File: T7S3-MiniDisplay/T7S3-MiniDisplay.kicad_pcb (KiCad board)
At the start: 2 copper layers, 67.3 x 63.5 mm, 37 parts, among them J101 Qwicc, J102 Micro_SD_Card_Det, J801 RJ45, J802 RJ45, T801 + 15 in -, T802 + 15 out -, U101 TTGO-T7_S3-V1.1, U301 AP63205, U801 TCAN332DR

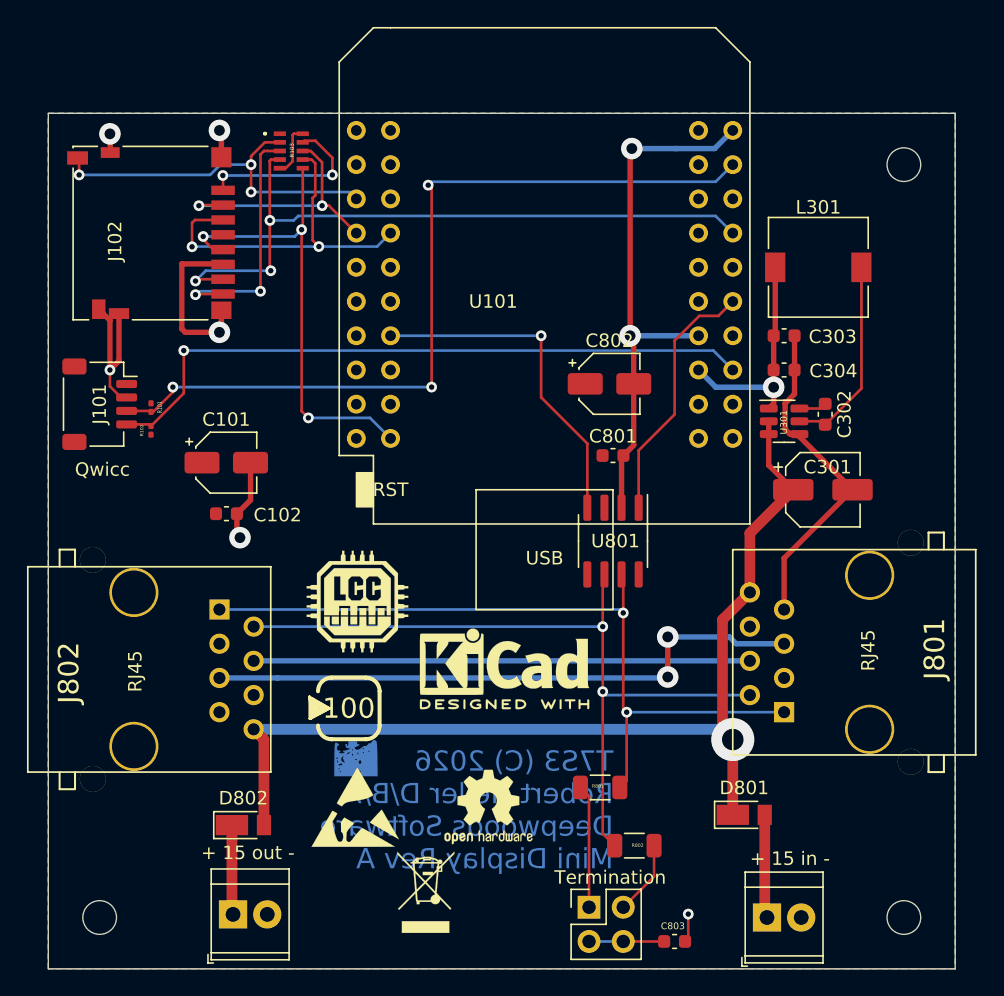
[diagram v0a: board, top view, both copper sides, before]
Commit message: Finalize part numbers.
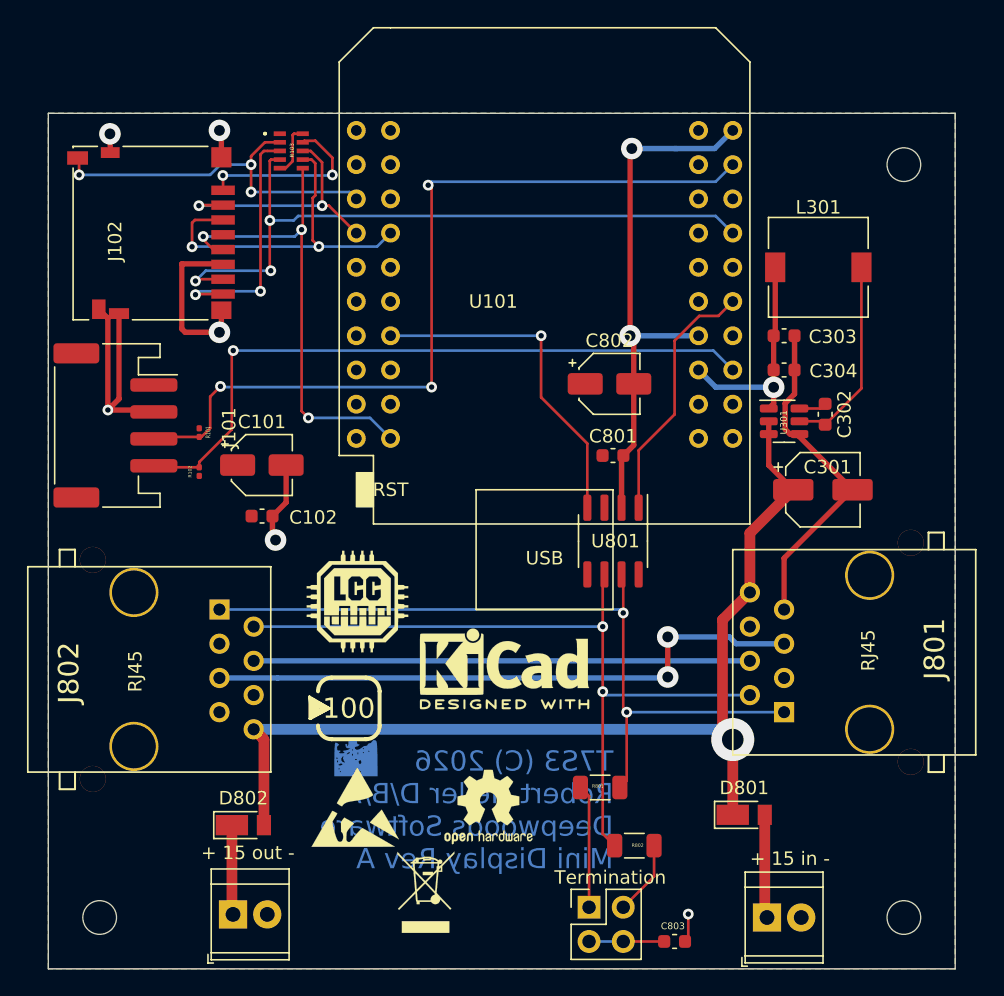
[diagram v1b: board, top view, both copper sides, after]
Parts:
- J101: footprint Connector_JST:JST_SH_SM04B-SRSS-TB_1x04-1MP_P1.00mm_Horizontal -> Connector_JST:JST_PH_S4B-PH-SM4-TB_1x04-1MP_P2.00mm_Horizontal
- moved R102 4.71 mm to (106.5, 58.3)
- moved R101 4.03 mm to (106.5, 55.4)
- moved C101 2.65 mm to (111.1, 57.9)
- moved C102 2.65 mm to (111.1, 61.6)
- moved J101 1.96 mm to (100.2, 54.9)
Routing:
- net GND: track 102.1 -> 108.7 mm
- net /SDA: track 49.8 -> 50.8 mm
